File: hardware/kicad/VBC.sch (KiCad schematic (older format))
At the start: 57 parts, among them J1 Conn_01x01, J10 Conn_01x01, J2 USB_OTG, J3 RJ25, J4 Conn_01x02, J5 RJ11, J6 RJ11, J7 RJ11, J8 RJ11, J9 USB_A, K1 RELAY_Metaltex, K2 RELAY_Metaltex, K3 RELAY_Metaltex, K4 RELAY_Metaltex, P1 CONN_01X01, Q1 BC817, Q2 BC817, Q3 BC817, Q4 BC817

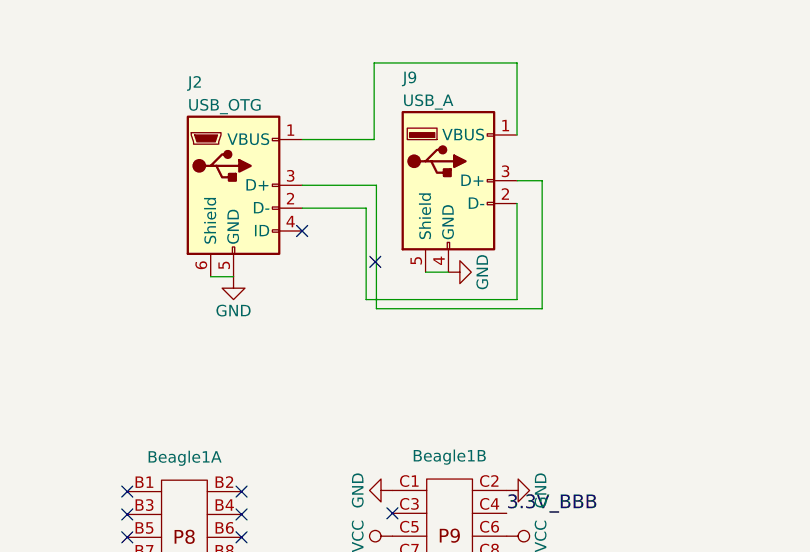
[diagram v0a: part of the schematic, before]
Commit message: new hardware version
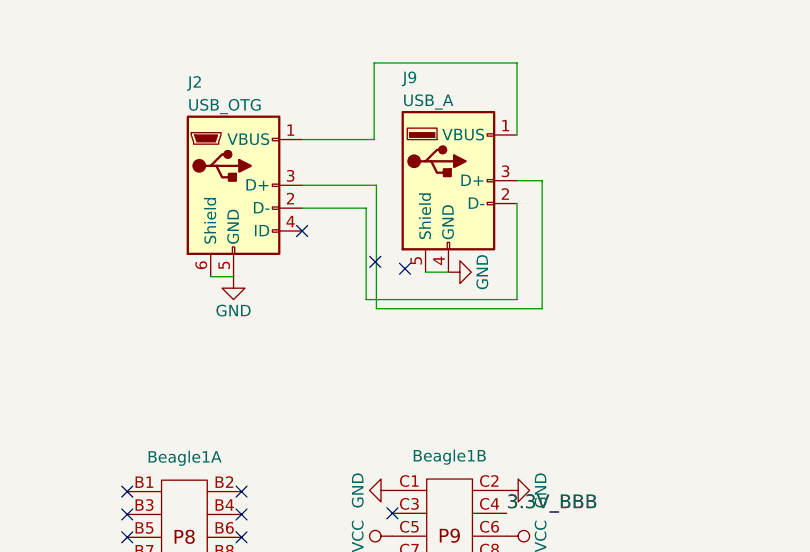
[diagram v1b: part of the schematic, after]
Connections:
- no-connect marks 89 -> 90
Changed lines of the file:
@@
 NoConn ~ 8950 2885
 NoConn ~ 8950 2985
+NoConn ~ 10165 1610
 $EndSCHEMATC
